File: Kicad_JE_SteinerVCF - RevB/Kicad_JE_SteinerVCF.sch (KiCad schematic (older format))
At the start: 72 parts, among them J101 HP, J102 BP, J103 LP, J104 Out, J105 CV, P101 Doepfer_Power_10pin, Q101 BC559, Q102 BC549, Q103 BC549, Q104 BC549

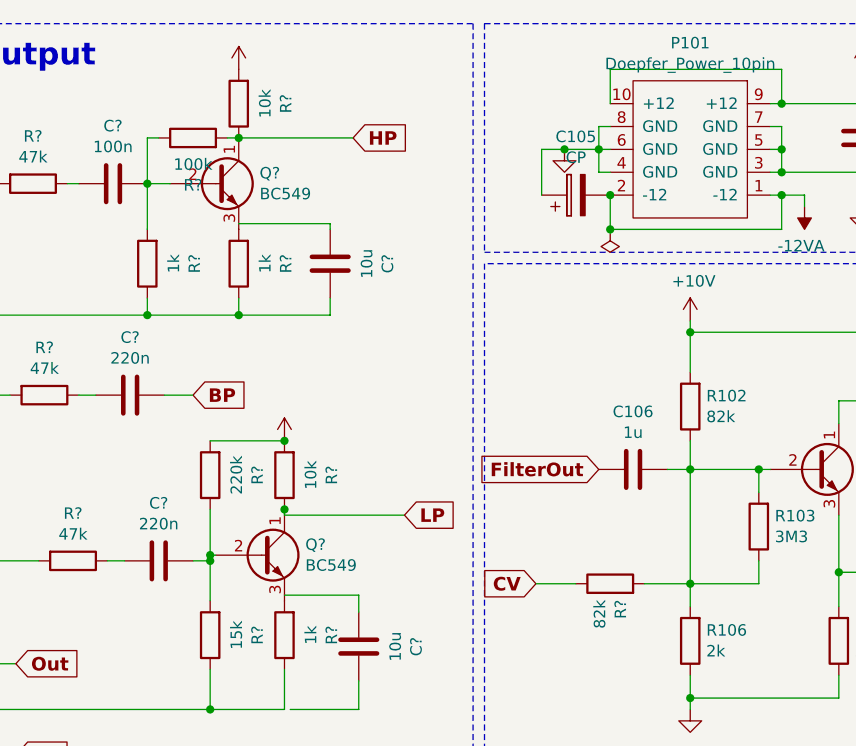
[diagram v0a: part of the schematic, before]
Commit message: fix reintroduced
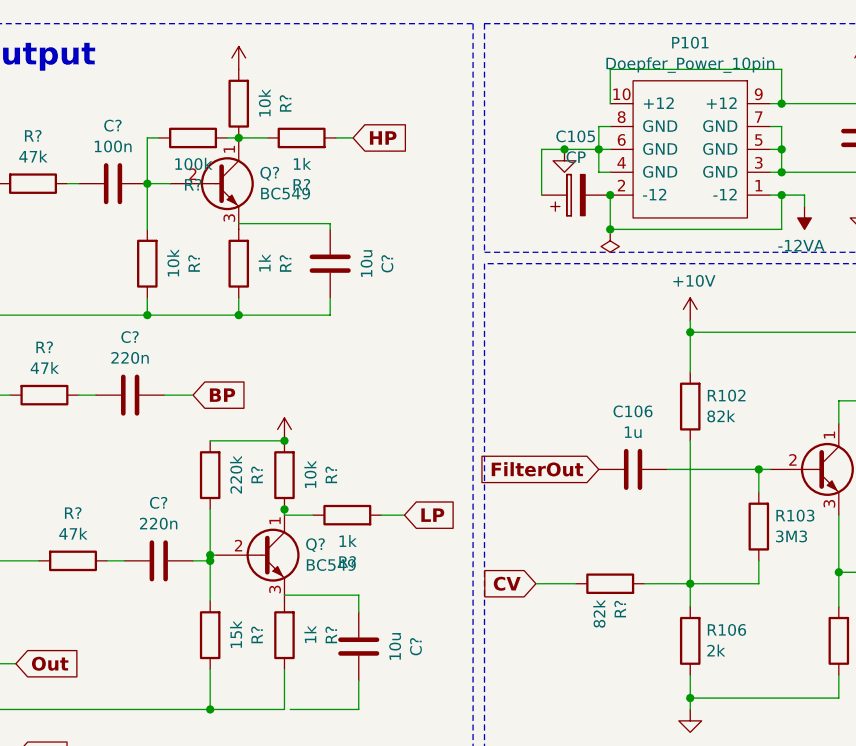
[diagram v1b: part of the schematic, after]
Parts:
- added R? (x2): 1k, Resistor_THT:R_Axial_DIN0309_L9.0mm_D3.2mm_P12.70mm_Horizontal, symbol Device:R
- R?: value 1k -> 10k
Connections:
- net HP: now also R?.2; no longer Q?.1 (C), R?.1, R?.2
- net LP: now also R?.2; no longer Q?.1 (C), R?.1
- net at R102.1, R103.1, R106.2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: no longer C106.1, Q102.2 (B), R103.2
- new net: C106.1, Q102.2 (B), R103.2
- new net: Q?.1 (C), R?.1, R?.1, R?.2
- new net: Q?.1 (C), R?.1, R?.1
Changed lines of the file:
@@
 JE-VCO1
 Wire Wire Line
-	4350 2425 4350 2550
-Wire Wire Line
 	4250 2550 4350 2550
-Wire Wire Line
-	4350 2550 4350 3050
 Text GLabel 3675 3050 0    59   Input ~ 12
 CV
@@
 Wire Wire Line
 	3675 3050 3850 3050
-Connection ~ 4350 2550
 Wire Wire Line
 	4350 2550 4650 2550
@@
 Connection ~ 2375 1875
 Wire Wire Line
-	2375 1100 2875 1100
-Wire Wire Line
-	2575 2750 3100 2750
+	2375 1100 2500 1100
+Wire Wire Line
+	2575 2750 2700 2750
 Connection ~ 3200 6150
 Wire Wire Line
@@
 P 1975 1650
 F 0 "R?" V 1768 1650 50  0000 C CNN
-F 1 "1k" V 1859 1650 50  0000 C CNN
+F 1 "10k" V 1859 1650 50  0000 C CNN
 F 2 "Resistor_THT:R_Axial_DIN0309_L9.0mm_D3.2mm_P12.70mm_Horizontal" V 1905 1650 50  0001 C CNN
 F 3 "~" H 1975 1650 50  0001 C CNN
@@
 Wire Wire Line
 	1975 1500 1975 1300
+$Comp
+L Device:R R?
+U 1 1 5CAAB3D3
+P 2850 2750
+F 0 "R?" V 2643 2750 50  0000 C CNN
+F 1 "1k" V 2734 2750 50  0000 C CNN
+F 2 "Resistor_THT:R_Axial_DIN0309_L9.0mm_D3.2mm_P12.70mm_Horizontal" V 2780 2750 50  0001 C CNN
+F 3 "~" H 2850 2750 50  0001 C CNN
+	1    2850 2750
+	0    -1   -1   0
+$EndComp
+Wire Wire Line
+	3000 2750 3100 2750
+$Comp
+L Device:R R?
+U 1 1 5CAAB50A
+P 2650 1100
+F 0 "R?" V 2443 1100 50  0000 C CNN
+F 1 "1k" V 2534 1100 50  0000 C CNN
+F 2 "Resistor_THT:R_Axial_DIN0309_L9.0mm_D3.2mm_P12.70mm_Horizontal" V 2580 1100 50  0001 C CNN
+F 3 "~" H 2650 1100 50  0001 C CNN
+	1    2650 1100
+	0    -1   -1   0
+$EndComp
+Wire Wire Line
+	2800 1100 2875 1100
+Wire Wire Line
+	4350 2425 4350 3050
 $EndSCHEMATC
